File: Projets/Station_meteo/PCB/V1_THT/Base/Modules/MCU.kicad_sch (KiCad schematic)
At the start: 9 parts, among them J1 Conn_02x05_Odd_Even, J2 Conn_02x04_Odd_Even, J3 Conn_02x06_Odd_Even, J4 Conn_02x06_Odd_Even, U1 ATmega328P-P, Y1 16 MHz HC49-4H

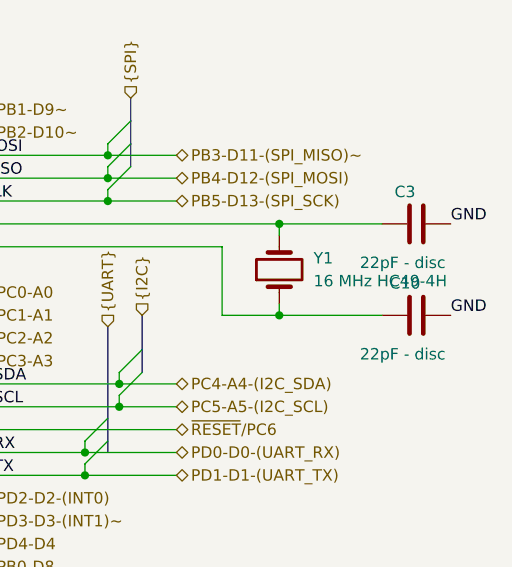
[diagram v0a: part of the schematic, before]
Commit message: Update Base
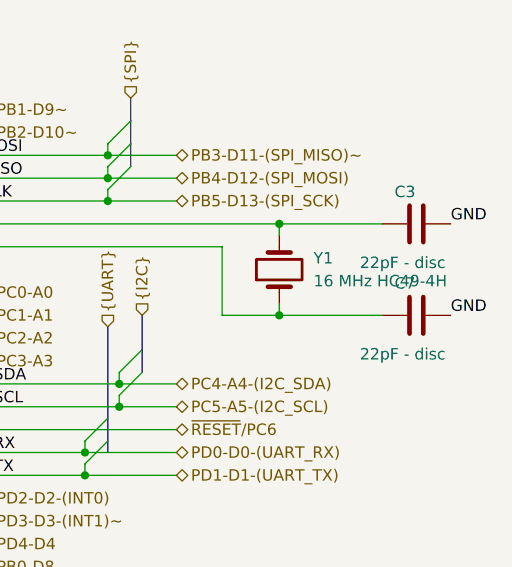
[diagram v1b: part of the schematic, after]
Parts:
- removed C10: 22pF - disc, Capacitor_THT:C_Radial_D5.0mm_H11.0mm_P2.00mm, symbol Device:C
- added C7: 22pF - disc, Capacitor_THT:C_Disc_D4.3mm_W1.9mm_P5.00mm, symbol Device:C
- C3: footprint Capacitor_THT:C_Radial_D5.0mm_H11.0mm_P2.00mm -> Capacitor_THT:C_Disc_D4.3mm_W1.9mm_P5.00mm
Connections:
- net GND: now also C7.2
- net at U1.10 (XTAL2/PB7), Y1.1: now also C7.1
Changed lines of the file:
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@@
 			)
 		)
-		(property "Footprint" "Capacitor_THT:C_Radial_D5.0mm_H11.0mm_P2.00mm"
+		(property "Footprint" "Capacitor_THT:C_Disc_D4.3mm_W1.9mm_P5.00mm"
 			(at 162.56 46.0248 0)
 			(effects
@@
 				(path "/4bc9f80e-0a24-4618-ba5d-3a118070c43e/6df9e135-6b30-40c1-b1f1-f69b9f79101d"
 					(reference "C3")
+					(unit 1)
+				)
+			)
+		)
+	)
+	(symbol
+		(lib_id "Device:C")
+		(at 158.75 57.15 90)
+		(unit 1)
+		(exclude_from_sim no)
+		(in_bom yes)
+		(on_board yes)
+		(dnp no)
+		(property "Reference" "C7"
+			(at 157.48 53.594 90)
+			(effects
+				(font
+					(size 1.27 1.27)
+				)
+			)
+		)
+		(property "Value" "22pF - disc"
+			(at 157.226 61.468 90)
+			(effects
+				(font
+					(size 1.27 1.27)
+				)
+			)
+		)
+		(property "Footprint" "Capacitor_THT:C_Disc_D4.3mm_W1.9mm_P5.00mm"
+			(at 162.56 56.1848 0)
+			(effects
+				(font
+					(size 1.27 1.27)
+				)
+				(hide yes)
+			)
+		)
+		(property "Datasheet" "~"
+			(at 158.75 57.15 0)
+			(effects
+				(font
+					(size 1.27 1.27)
+				)
+				(hide yes)
+			)
+		)
+		(property "Description" "Unpolarized capacitor"
+			(at 158.75 57.15 0)
+			(effects
+				(font
+					(size 1.27 1.27)
+				)
+				(hide yes)
+			)
+		)
+		(pin "2"
+		)
+		(pin "1"
+		)
+		(instances
+			(project "Base"
+				(path "/4bc9f80e-0a24-4618-ba5d-3a118070c43e/6df9e135-6b30-40c1-b1f1-f69b9f79101d"
+					(reference "C7")
 					(unit 1)
 				)
@@
 					(unit 1)
 				)
-			)
-		)
-	)
-	(symbol
-		(lib_id "Device:C")
-		(at 158.75 57.15 90)
-		(unit 1)
-		(exclude_from_sim no)
-		(in_bom yes)
-		(on_board yes)
-		(dnp no)
-		(property "Reference" "C10"
-			(at 157.48 53.594 90)
-			(effects
-				(font
-					(size 1.27 1.27)
-				)
-			)
-		)
-		(property "Value" "22pF - disc"
-			(at 157.226 61.468 90)
-			(effects
-				(font
-					(size 1.27 1.27)
-				)
-			)
-		)
-		(property "Footprint" "Capacitor_THT:C_Radial_D5.0mm_H11.0mm_P2.00mm"
-			(at 162.56 56.1848 0)
-			(effects
-				(font
-					(size 1.27 1.27)
-				)
-				(hide yes)
-			)
-		)
-		(property "Datasheet" "~"
-			(at 158.75 57.15 0)
-			(effects
-				(font
-					(size 1.27 1.27)
-				)
-				(hide yes)
-			)
-		)
-		(property "Description" "Unpolarized capacitor"
-			(at 158.75 57.15 0)
-			(effects
-				(font
-					(size 1.27 1.27)
-				)
-				(hide yes)
-			)
-		)
-		(pin "2"
-		)
-		(pin "1"
-		)
-		(instances
-			(project "Base"
-				(path "/4bc9f80e-0a24-4618-ba5d-3a118070c43e/6df9e135-6b30-40c1-b1f1-f69b9f79101d"
-					(reference "C10")
-					(unit 1)
-				)
